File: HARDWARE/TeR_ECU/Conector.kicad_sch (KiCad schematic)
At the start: 1 part, among them IC1 MX34040NF2

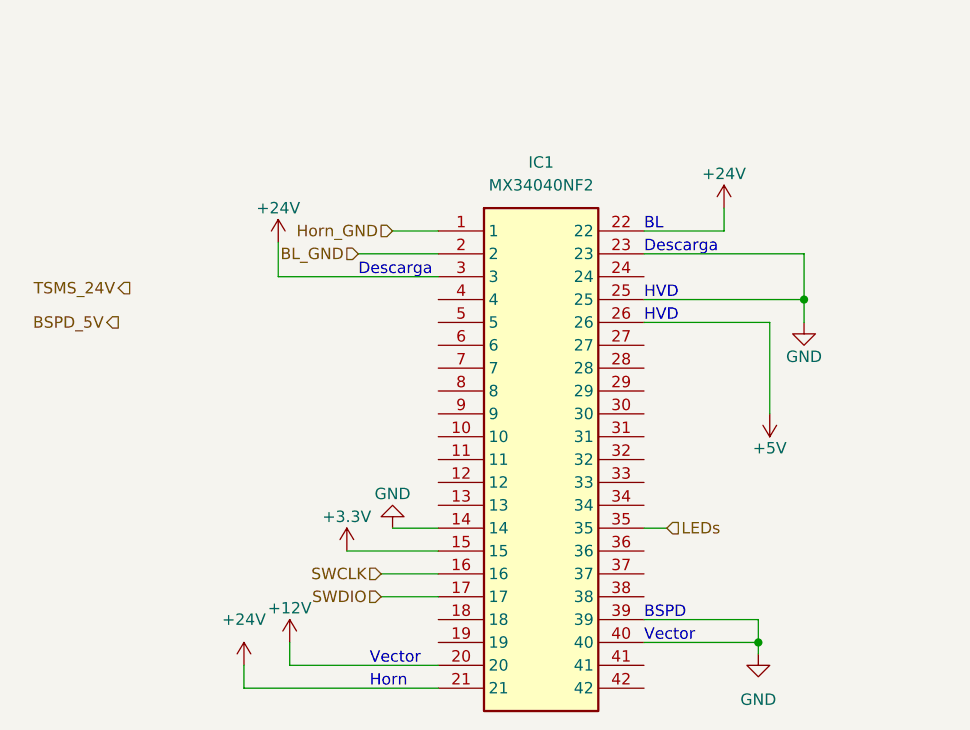
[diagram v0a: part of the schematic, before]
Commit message: Solo falta revisar
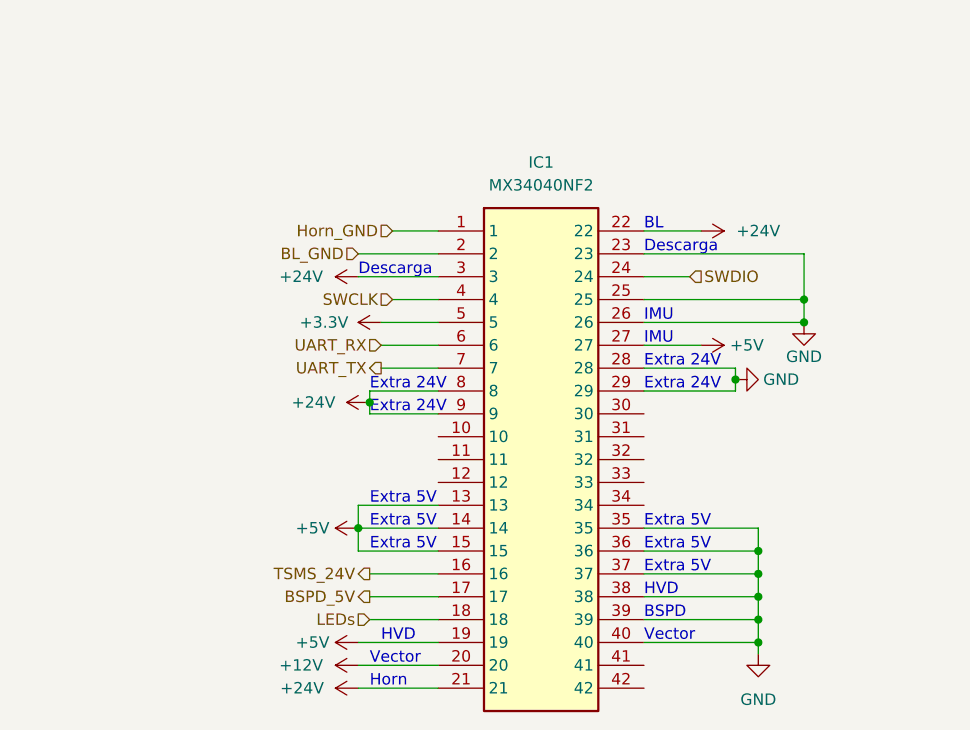
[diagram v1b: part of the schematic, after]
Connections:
- net +24V: now also IC1.8, IC1.9
- net +3.3V: now also IC1.5; no longer IC1.15
- net +5V: now also IC1.13, IC1.14, IC1.15, IC1.19, IC1.27; no longer IC1.26
- net BSPD_5V: now also IC1.17
- net GND: now also IC1.26, IC1.28, IC1.29, IC1.35, IC1.36, IC1.37, IC1.38; no longer IC1.14
- net LEDs: now also IC1.18; no longer IC1.35
- net SWCLK: now also IC1.4; no longer IC1.16
- net SWDIO: now also IC1.24; no longer IC1.17
- net TSMS_24V: now also IC1.16
- net UART_RX: now reaches IC1.6
- net UART_TX: now reaches IC1.7
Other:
- note added: "Extra 24V"
- note added: "Extra 5V"
- note added: "IMU"
